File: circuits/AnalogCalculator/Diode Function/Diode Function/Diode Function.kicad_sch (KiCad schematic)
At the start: 69 parts, among them J1 Conn_01x08_Pin

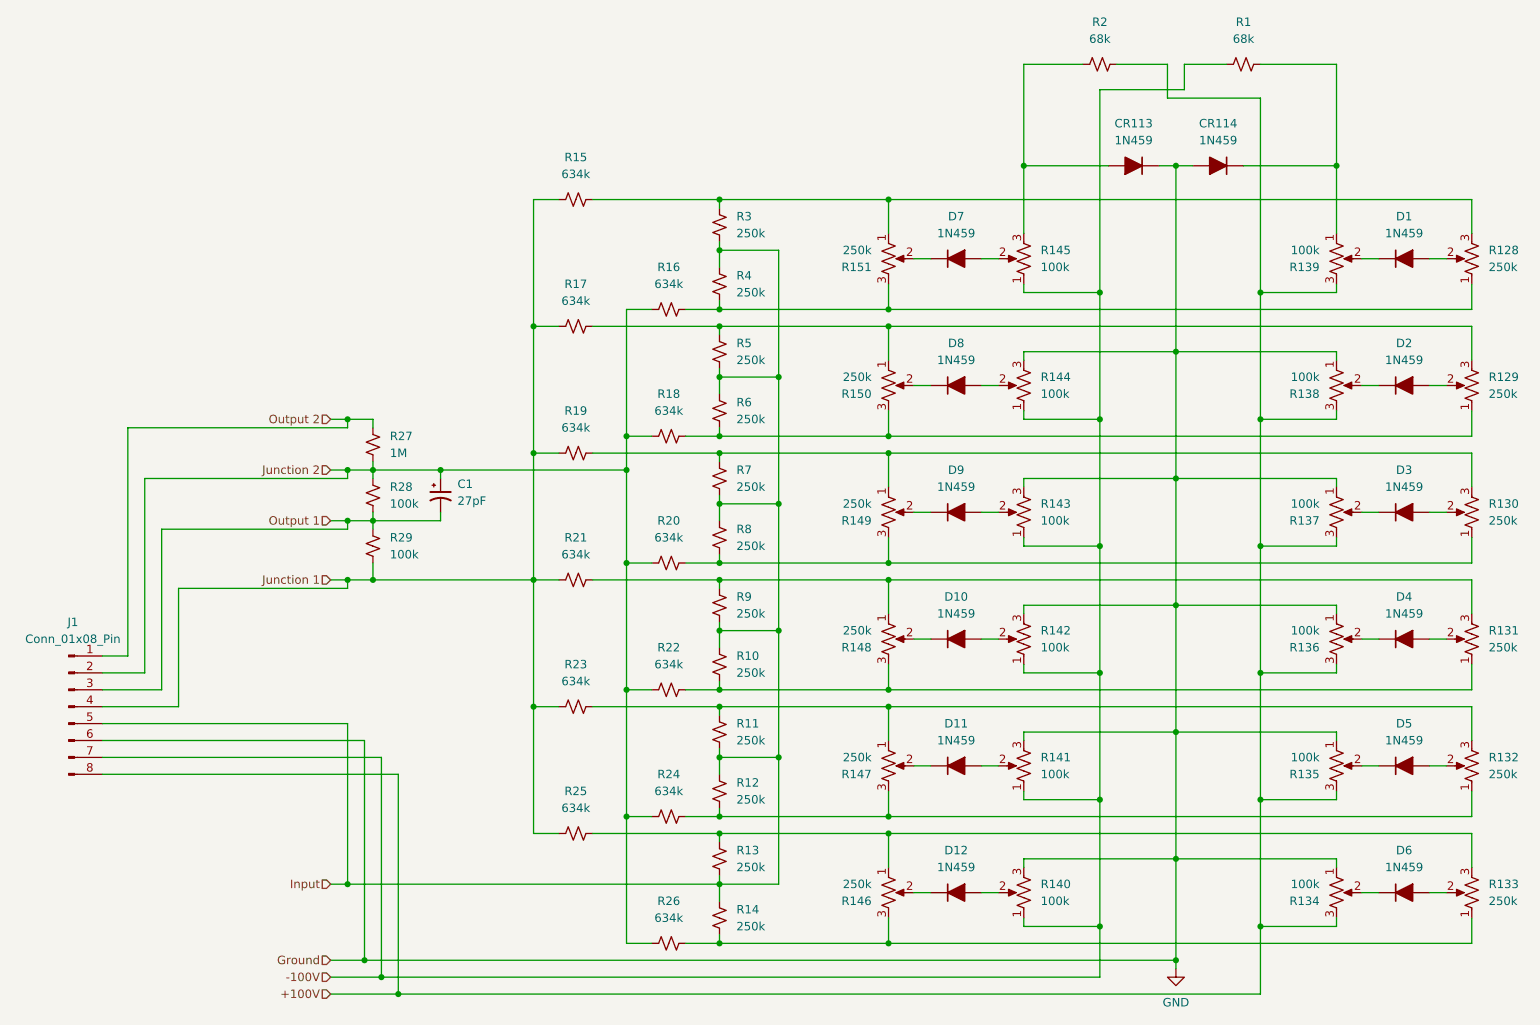
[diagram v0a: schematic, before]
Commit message: update notes
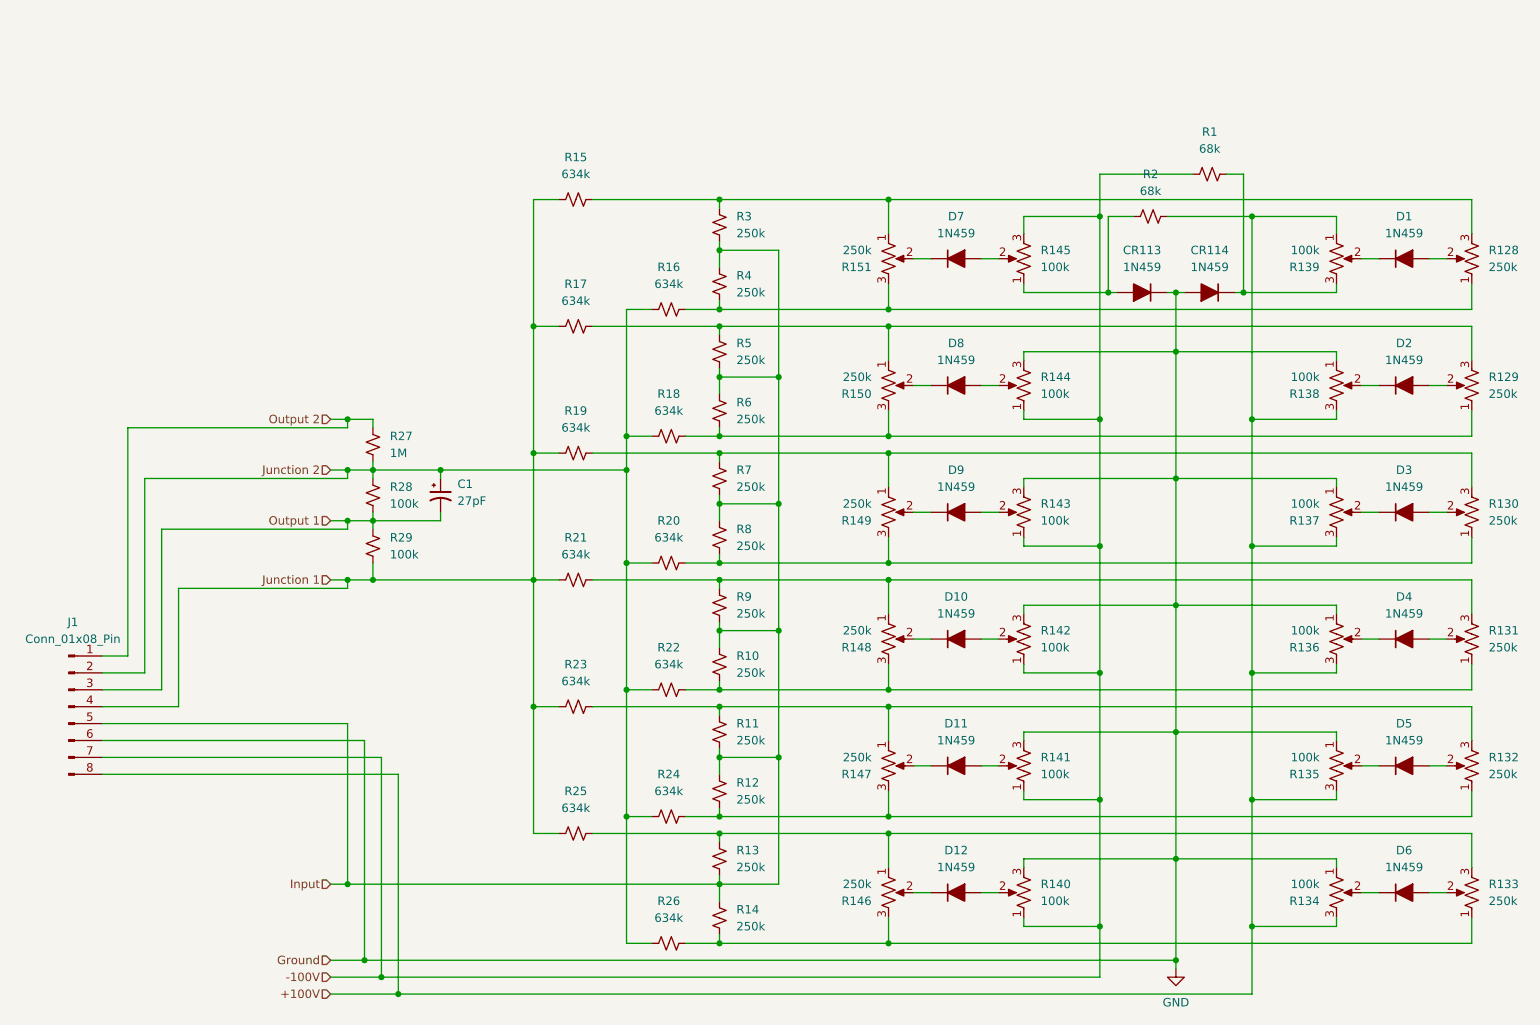
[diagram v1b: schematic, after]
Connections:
- net +100V: now also R139.1; no longer R139.3
- net -100V: now also R145.3; no longer R145.1
- net at CR113.2 (A), R2.1: now also R145.1; no longer R145.3
- net at CR114.1 (K), R1.2: now also R139.3; no longer R139.1
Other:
- moved on the sheet: CR113, CR114, R1, R2
